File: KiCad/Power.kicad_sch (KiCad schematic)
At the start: 32 parts, among them J7 Screw_Terminal_01x02, J8 Screw_Terminal_01x02, J9 Screw_Terminal_01x02, U14 L298P, U5 LM1117DT-3.3, U6 LM2596T-5

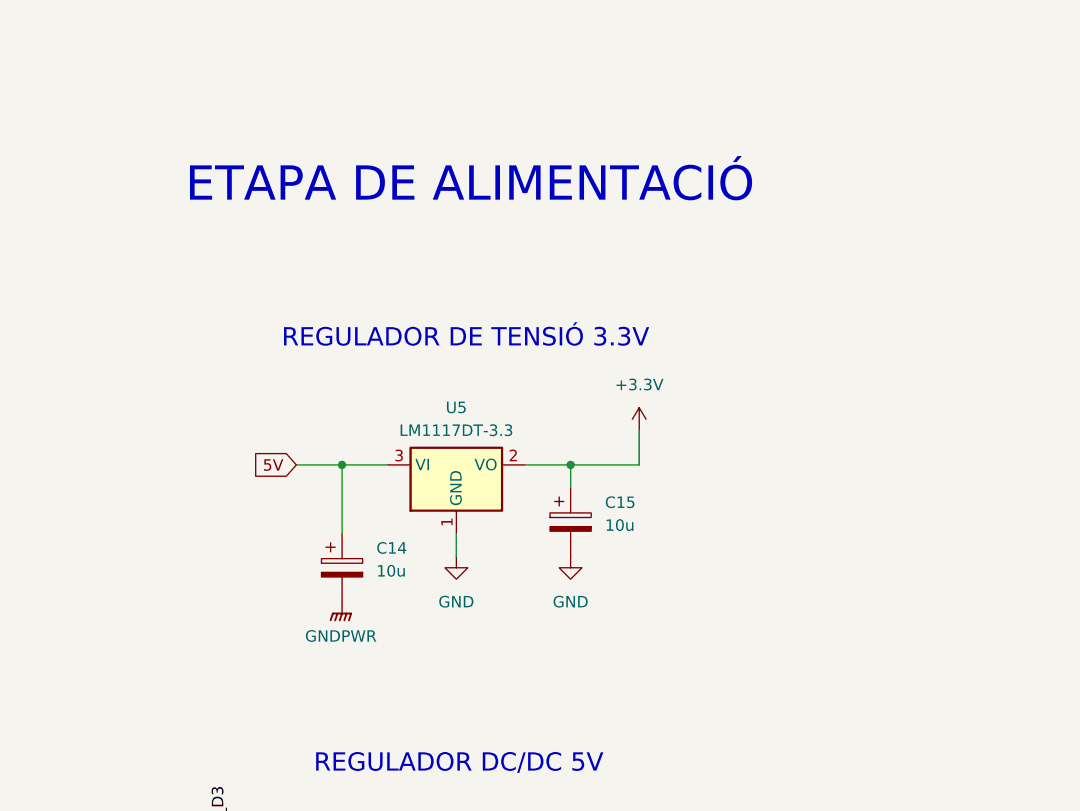
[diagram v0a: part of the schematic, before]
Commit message: Sensor Hall y LED mas o menos definitivos
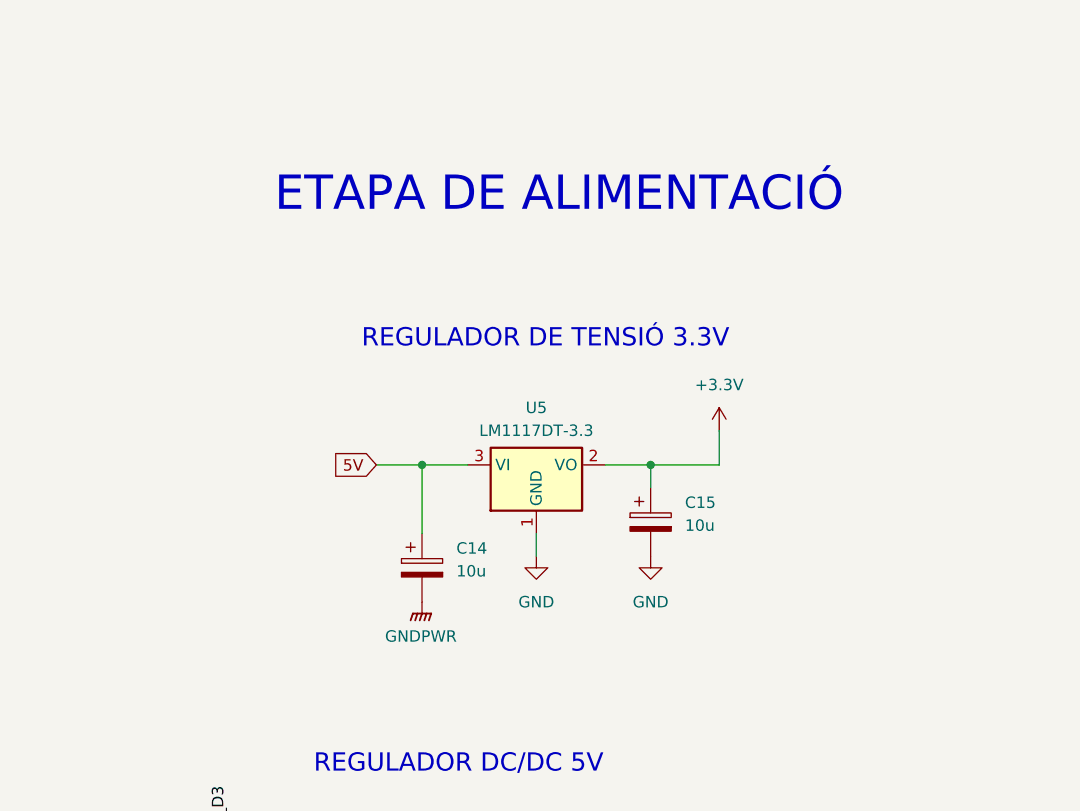
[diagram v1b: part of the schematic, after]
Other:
- moved on the sheet: C14, C15, U5
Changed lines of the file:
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@@
 	(text "ETAPA DE ALIMENTACIÓ\n"
 		(exclude_from_sim no)
-		(at 66.294 52.832 0)
+		(at 76.2 53.848 0)
 		(effects
 			(font
@@
 	(text "REGULADOR DE TENSIÓ 3.3V\n"
 		(exclude_from_sim no)
-		(at 65.786 69.85 0)
+		(at 74.676 69.85 0)
 		(effects
 			(font
@@
 	)
 	(junction
-		(at 52.07 83.82)
+		(at 60.96 83.82)
 		(diameter 0)
 		(color 0 0 0 0)
 	)
 	(junction
-		(at 77.47 83.82)
+		(at 86.36 83.82)
 		(diameter 0)
 		(color 0 0 0 0)
@@
 	(wire
 		(pts
-			(xy 52.07 83.82) (xy 57.15 83.82)
+			(xy 60.96 83.82) (xy 66.04 83.82)
 		)
 		(stroke
@@
 	(wire
 		(pts
-			(xy 85.09 80.01) (xy 85.09 83.82)
+			(xy 93.98 80.01) (xy 93.98 83.82)
 		)
 		(stroke
@@
 	(wire
 		(pts
-			(xy 77.47 83.82) (xy 77.47 86.36)
+			(xy 86.36 83.82) (xy 86.36 86.36)
 		)
 		(stroke
@@
 	(wire
 		(pts
-			(xy 72.39 83.82) (xy 77.47 83.82)
+			(xy 81.28 83.82) (xy 86.36 83.82)
 		)
 		(stroke
@@
 	(wire
 		(pts
-			(xy 64.77 91.44) (xy 64.77 93.98)
+			(xy 73.66 91.44) (xy 73.66 93.98)
 		)
 		(stroke
@@
 	(wire
 		(pts
-			(xy 52.07 83.82) (xy 52.07 91.44)
+			(xy 60.96 83.82) (xy 60.96 91.44)
 		)
 		(stroke
@@
 	(wire
 		(pts
-			(xy 77.47 83.82) (xy 85.09 83.82)
+			(xy 86.36 83.82) (xy 93.98 83.82)
 		)
 		(stroke
@@
 	(wire
 		(pts
-			(xy 46.99 83.82) (xy 52.07 83.82)
+			(xy 55.88 83.82) (xy 60.96 83.82)
 		)
 		(stroke
@@
 	(global_label "5V"
 		(shape input)
-		(at 46.99 83.82 180)
+		(at 55.88 83.82 180)
 		(fields_autoplaced yes)
 		(effects
@@
 		)
 		(property "Intersheetrefs" "${INTERSHEET_REFS}"
-			(at 41.7067 83.82 0)
+			(at 50.5967 83.82 0)
 			(effects
 				(font
@@
 	(symbol
 		(lib_id "Regulator_Linear:LM1117DT-3.3")
-		(at 64.77 83.82 0)
+		(at 73.66 83.82 0)
 		(unit 1)
 		(exclude_from_sim no)
@@
 		(fields_autoplaced yes)
 		(property "Reference" "U5"
-			(at 64.77 77.47 0)
+			(at 73.66 77.47 0)
 			(effects
 				(font
@@
 		)
 		(property "Value" "LM1117DT-3.3"
-			(at 64.77 80.01 0)
+			(at 73.66 80.01 0)
 			(effects
 				(font
@@
 		)
 		(property "Footprint" "Package_TO_SOT_SMD:TO-252-3_TabPin2"
-			(at 64.77 83.82 0)
+			(at 73.66 83.82 0)
 			(effects
 				(font
@@
 		)
 		(property "Datasheet" "http://www.ti.com/lit/ds/symlink/lm1117.pdf"
-			(at 64.77 83.82 0)
+			(at 73.66 83.82 0)
 			(effects
 				(font
@@
 		)
 		(property "Description" "800mA Low-Dropout Linear Regulator, 3.3V fixed output, TO-252"
-			(at 64.77 83.82 0)
+			(at 73.66 83.82 0)
 			(effects
 				(font
@@
 	(symbol
 		(lib_id "Device:C_Polarized")
-		(at 52.07 95.25 0)
+		(at 60.96 95.25 0)
 		(unit 1)
 		(exclude_from_sim no)
@@
 		(fields_autoplaced yes)
 		(property "Reference" "C14"
-			(at 55.88 93.0909 0)
+			(at 64.77 93.0909 0)
 			(effects
 				(font
@@
 		)
 		(property "Value" "10u"
-			(at 55.88 95.6309 0)
+			(at 64.77 95.6309 0)
 			(effects
 				(font
@@
 		)
 		(property "Footprint" "Capacitor_SMD:C_0805_2012Metric"
-			(at 53.0352 99.06 0)
+			(at 61.9252 99.06 0)
 			(effects
 				(font
@@
 		)
 		(property "Datasheet" "~"
-			(at 52.07 95.25 0)
+			(at 60.96 95.25 0)
 			(effects
 				(font
@@
 		)
 		(property "Description" "Polarized capacitor"
-			(at 52.07 95.25 0)
+			(at 60.96 95.25 0)
 			(effects
 				(font
@@
 	(symbol
 		(lib_id "Device:C_Polarized")
-		(at 77.47 90.17 0)
+		(at 86.36 90.17 0)
 		(unit 1)
 		(exclude_from_sim no)
@@
 		(fields_autoplaced yes)
 		(property "Reference" "C15"
-			(at 81.28 88.0109 0)
+			(at 90.17 88.0109 0)
 			(effects
 				(font
@@
 		)
 		(property "Value" "10u"
-			(at 81.28 90.5509 0)
+			(at 90.17 90.5509 0)
 			(effects
 				(font
@@
 		)
 		(property "Footprint" "Capacitor_SMD:C_0805_2012Metric"
-			(at 78.4352 93.98 0)
+			(at 87.3252 93.98 0)
 			(effects
 				(font
@@
 		)
 		(property "Datasheet" "~"
-			(at 77.47 90.17 0)
+			(at 86.36 90.17 0)
 			(effects
 				(font
@@
 		)
 		(property "Description" "Polarized capacitor"
-			(at 77.47 90.17 0)
+			(at 86.36 90.17 0)
 			(effects
 				(font
@@
 	(symbol
 		(lib_id "power:+3.3V")
-		(at 85.09 80.01 0)
+		(at 93.98 80.01 0)
 		(unit 1)
 		(exclude_from_sim no)
@@
 		(fields_autoplaced yes)
 		(property "Reference" "#PWR037"
-			(at 85.09 83.82 0)
+			(at 93.98 83.82 0)
 			(effects
 				(font
@@
 		)
 		(property "Value" "+3.3V"
-			(at 85.09 74.93 0)
+			(at 93.98 74.93 0)
 			(effects
 				(font
@@
 		)
 		(property "Footprint" ""
-			(at 85.09 80.01 0)
+			(at 93.98 80.01 0)
 			(effects
 				(font
@@
 		)
 		(property "Datasheet" ""
-			(at 85.09 80.01 0)
+			(at 93.98 80.01 0)
 			(effects
 				(font
@@
 		)
 		(property "Description" "Power symbol creates a global label with name \"+3.3V\""
-			(at 85.09 80.01 0)
+			(at 93.98 80.01 0)
 			(effects
 				(font
@@
 	(symbol
 		(lib_id "power:GND")
-		(at 77.47 93.98 0)
+		(at 86.36 93.98 0)
 		(unit 1)
 		(exclude_from_sim no)
@@
 		(fields_autoplaced yes)
 		(property "Reference" "#PWR033"
-			(at 77.47 100.33 0)
+			(at 86.36 100.33 0)
 			(effects
 				(font
@@
 		)
 		(property "Value" "GND"
-			(at 77.47 99.06 0)
+			(at 86.36 99.06 0)
 			(effects
 				(font
@@
 		)
 		(property "Footprint" ""
-			(at 77.47 93.98 0)
+			(at 86.36 93.98 0)
 			(effects
 				(font
@@
 		)
 		(property "Datasheet" ""
-			(at 77.47 93.98 0)
+			(at 86.36 93.98 0)
 			(effects
 				(font
@@
 		)
 		(property "Description" "Power symbol creates a global label with name \"GND\" , ground"
-			(at 77.47 93.98 0)
+			(at 86.36 93.98 0)
 			(effects
 				(font
@@
 	(symbol
 		(lib_id "power:GND")
-		(at 64.77 93.98 0)
+		(at 73.66 93.98 0)
 		(unit 1)
 		(exclude_from_sim no)
@@
 		(fields_autoplaced yes)
 		(property "Reference" "#PWR034"
-			(at 64.77 100.33 0)
+			(at 73.66 100.33 0)
 			(effects
 				(font
@@
 		)
 		(property "Value" "GND"
-			(at 64.77 99.06 0)
+			(at 73.66 99.06 0)
 			(effects
 				(font
@@
 		)
 		(property "Footprint" ""
-			(at 64.77 93.98 0)
+			(at 73.66 93.98 0)
 			(effects
 				(font
@@
 		)
 		(property "Datasheet" ""
-			(at 64.77 93.98 0)
+			(at 73.66 93.98 0)
 			(effects
 				(font
@@
 		)
 		(property "Description" "Power symbol creates a global label with name \"GND\" , ground"
-			(at 64.77 93.98 0)
+			(at 73.66 93.98 0)
 			(effects
 				(font
@@
 	(symbol
 		(lib_id "power:GNDPWR")
-		(at 52.07 99.06 0)
+		(at 60.96 99.06 0)
 		(unit 1)
 		(exclude_from_sim no)
@@
 		(fields_autoplaced yes)
 		(property "Reference" "#PWR058"
-			(at 52.07 104.14 0)
+			(at 60.96 104.14 0)
 			(effects
 				(font
@@
 		)
 		(property "Value" "GNDPWR"
-			(at 51.943 102.87 0)
+			(at 60.833 102.87 0)
 			(effects
 				(font
@@
 		)
 		(property "Footprint" ""
-			(at 52.07 100.33 0)
+			(at 60.96 100.33 0)
 			(effects
 				(font
@@
 		)
 		(property "Datasheet" ""
-			(at 52.07 100.33 0)
+			(at 60.96 100.33 0)
 			(effects
 				(font
@@
 		)
 		(property "Description" "Power symbol creates a global label with name \"GNDPWR\" , global ground"
-			(at 52.07 99.06 0)
+			(at 60.96 99.06 0)
 			(effects
 				(font
